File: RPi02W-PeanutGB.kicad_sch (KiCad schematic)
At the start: 64 parts, among them J1 Raspberry_Pi_2_3, J3 AudioJack3_SwitchTR, J4 Conn_01x50, J5 Conn_02x10_Odd_Even, J6 Conn_02x10_Odd_Even, J7 Conn_02x10_Odd_Even, J8 Conn_02x10_Odd_Even, J9 USB_C_Receptacle, SW1 SW_SPDT_MSM, SW10 SW_Push, SW11 SW_Push, SW12 SW_Push, SW13 SW_Push, SW14 SW_Push, SW2 SW_Push, SW3 SW_Push, SW4 SW_Push, SW5 SW_Push, SW6 SW_Push, SW7 SW_Push, SW8 SW_Push, SW9 SW_Push, U1 MCP73831-2-OT, U3 LM4861MX

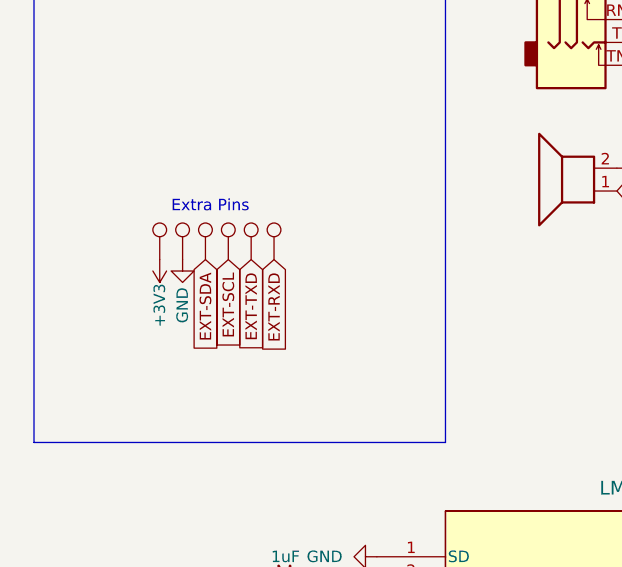
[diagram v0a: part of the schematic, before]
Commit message: Add files via upload
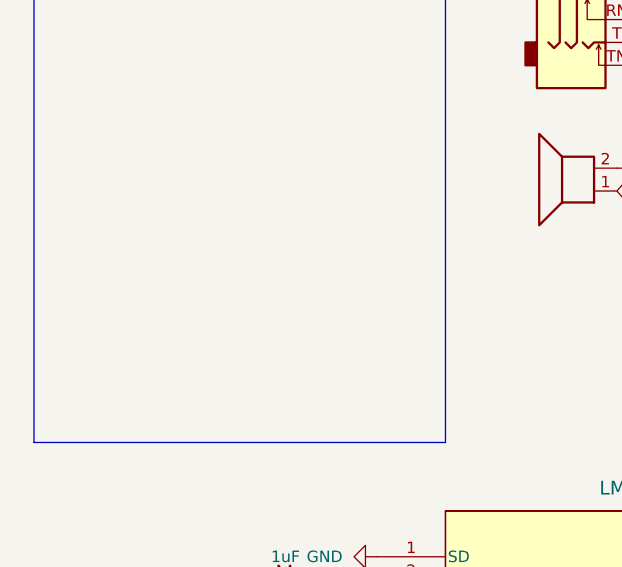
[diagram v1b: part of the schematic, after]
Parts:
- removed TP10, TP11, TP12, TP5, TP7, TP9: TestPoint, RPi02W-PeanutGB:TestPoint_THTPad_Edit_D1.5mm_Drill0.7mm, symbol Connector:TestPoint
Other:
- note removed: "Extra Pins"
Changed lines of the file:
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@@
     (effects (font (size 1.27 1.27)) (justify left bottom))
   )
-  (text "Extra Pins" (at 33.02 83.82 0)
-    (effects (font (size 1.27 1.27)) (justify left bottom))
-  )
   (global_label "BUTTON-DR" (shape input) (at 118.11 171.45 0) (fields_autoplaced)
     (effects (font (size 1.27 1.27)) (justify left))
@@
     )
   )
-  (global_label "EXT-SDA" (shape input) (at 36.83 88.9 270) (fields_autoplaced)
-    (effects (font (size 1.27 1.27)) (justify right))
-    (property "Intersheetrefs" "${INTERSHEET_REFS}" (at 36.83 100.3518 90)
-      (effects (font (size 1.27 1.27)) (justify right) hide)
-    )
-  )
   (global_label "BUTTON-B" (shape input) (at 195.58 22.86 0) (fields_autoplaced)
     (effects (font (size 1.27 1.27)) (justify left))
@@
     )
   )
-  (global_label "EXT-TXD" (shape input) (at 41.91 88.9 270) (fields_autoplaced)
-    (effects (font (size 1.27 1.27)) (justify right))
-    (property "Intersheetrefs" "${INTERSHEET_REFS}" (at 41.91 100.2308 90)
-      (effects (font (size 1.27 1.27)) (justify right) hide)
-    )
-  )
   (global_label "LCD-MOSI" (shape input) (at 217.17 181.61 180) (fields_autoplaced)
     (effects (font (size 1.27 1.27)) (justify right))
@@
     )
   )
-  (global_label "EXT-RXD" (shape input) (at 44.45 88.9 270) (fields_autoplaced)
-    (effects (font (size 1.27 1.27)) (justify right))
-    (property "Intersheetrefs" "${INTERSHEET_REFS}" (at 44.45 100.5332 90)
-      (effects (font (size 1.27 1.27)) (justify right) hide)
-    )
-  )
   (global_label "AUDIO-SPEAKER" (shape input) (at 82.55 81.28 0) (fields_autoplaced)
     (effects (font (size 1.27 1.27)) (justify left))
@@
     )
   )
-  (global_label "EXT-SCL" (shape input) (at 39.37 88.9 270) (fields_autoplaced)
-    (effects (font (size 1.27 1.27)) (justify right))
-    (property "Intersheetrefs" "${INTERSHEET_REFS}" (at 39.37 100.2913 90)
-      (effects (font (size 1.27 1.27)) (justify right) hide)
-    )
-  )
   (global_label "BUTTON-DL" (shape input) (at 57.15 171.45 180) (fields_autoplaced)
     (effects (font (size 1.27 1.27)) (justify right))
@@
     (property "Intersheetrefs" "${INTERSHEET_REFS}" (at 202.8757 176.53 0)
       (effects (font (size 1.27 1.27)) (justify right) hide)
-    )
-  )
-  (symbol (lib_id "Connector:TestPoint") (at 44.45 88.9 0) (unit 1)
-    (in_bom yes) (on_board yes) (dnp no) (fields_autoplaced)
-    (property "Reference" "TP12" (at 46.99 84.328 0)
-      (effects (font (size 1.27 1.27)) (justify left) hide)
-    )
-    (property "Value" "TestPoint" (at 46.99 86.868 0)
-      (effects (font (size 1.27 1.27)) (justify left) hide)
-    )
-    (property "Footprint" "RPi02W-PeanutGB:TestPoint_THTPad_Edit_D1.5mm_Drill0.7mm" (at 49.53 88.9 0)
-      (effects (font (size 1.27 1.27)) hide)
-    )
-    (property "Datasheet" "~" (at 49.53 88.9 0)
-      (effects (font (size 1.27 1.27)) hide)
-    )
-    (pin "1")
-    (instances
-      (project "RPi02W-PeanutGB"
-        (path "/4ab622d7-b3cd-4c8b-9519-077cc9b8f532"
-          (reference "TP12") (unit 1)
-        )
-      )
-    )
-  )
-  (symbol (lib_id "Connector:TestPoint") (at 31.75 88.9 0) (unit 1)
-    (in_bom yes) (on_board yes) (dnp no) (fields_autoplaced)
-    (property "Reference" "TP5" (at 34.29 84.328 0)
-      (effects (font (size 1.27 1.27)) (justify left) hide)
-    )
-    (property "Value" "TestPoint" (at 34.29 86.868 0)
-      (effects (font (size 1.27 1.27)) (justify left) hide)
-    )
-    (property "Footprint" "RPi02W-PeanutGB:TestPoint_THTPad_Edit_D1.5mm_Drill0.7mm" (at 36.83 88.9 0)
-      (effects (font (size 1.27 1.27)) hide)
-    )
-    (property "Datasheet" "~" (at 36.83 88.9 0)
-      (effects (font (size 1.27 1.27)) hide)
-    )
-    (pin "1")
-    (instances
-      (project "RPi02W-PeanutGB"
-        (path "/4ab622d7-b3cd-4c8b-9519-077cc9b8f532"
-          (reference "TP5") (unit 1)
-        )
-      )
     )
   )
@@
         (path "/4ab622d7-b3cd-4c8b-9519-077cc9b8f532"
           (reference "#PWR01") (unit 1)
-        )
-      )
-    )
-  )
-  (symbol (lib_id "Connector:TestPoint") (at 41.91 88.9 0) (unit 1)
-    (in_bom yes) (on_board yes) (dnp no) (fields_autoplaced)
-    (property "Reference" "TP11" (at 44.45 84.328 0)
-      (effects (font (size 1.27 1.27)) (justify left) hide)
-    )
-    (property "Value" "TestPoint" (at 44.45 86.868 0)
-      (effects (font (size 1.27 1.27)) (justify left) hide)
-    )
-    (property "Footprint" "RPi02W-PeanutGB:TestPoint_THTPad_Edit_D1.5mm_Drill0.7mm" (at 46.99 88.9 0)
-      (effects (font (size 1.27 1.27)) hide)
-    )
-    (property "Datasheet" "~" (at 46.99 88.9 0)
-      (effects (font (size 1.27 1.27)) hide)
-    )
-    (pin "1")
-    (instances
-      (project "RPi02W-PeanutGB"
-        (path "/4ab622d7-b3cd-4c8b-9519-077cc9b8f532"
-          (reference "TP11") (unit 1)
         )
       )
@@
     )
   )
-  (symbol (lib_id "Connector:TestPoint") (at 34.29 88.9 0) (unit 1)
-    (in_bom yes) (on_board yes) (dnp no) (fields_autoplaced)
-    (property "Reference" "TP7" (at 36.83 84.328 0)
-      (effects (font (size 1.27 1.27)) (justify left) hide)
-    )
-    (property "Value" "TestPoint" (at 36.83 86.868 0)
-      (effects (font (size 1.27 1.27)) (justify left) hide)
-    )
-    (property "Footprint" "RPi02W-PeanutGB:TestPoint_THTPad_Edit_D1.5mm_Drill0.7mm" (at 39.37 88.9 0)
-      (effects (font (size 1.27 1.27)) hide)
-    )
-    (property "Datasheet" "~" (at 39.37 88.9 0)
-      (effects (font (size 1.27 1.27)) hide)
-    )
-    (pin "1")
-    (instances
-      (project "RPi02W-PeanutGB"
-        (path "/4ab622d7-b3cd-4c8b-9519-077cc9b8f532"
-          (reference "TP7") (unit 1)
-        )
-      )
-    )
-  )
   (symbol (lib_id "Device:R_US") (at 247.65 35.56 90) (unit 1)
     (in_bom yes) (on_board yes) (dnp no)
@@
         (path "/4ab622d7-b3cd-4c8b-9519-077cc9b8f532"
           (reference "R8") (unit 1)
-        )
-      )
-    )
-  )
-  (symbol (lib_id "Connector:TestPoint") (at 39.37 88.9 0) (unit 1)
-    (in_bom yes) (on_board yes) (dnp no) (fields_autoplaced)
-    (property "Reference" "TP10" (at 41.91 84.328 0)
-      (effects (font (size 1.27 1.27)) (justify left) hide)
-    )
-    (property "Value" "TestPoint" (at 41.91 86.868 0)
-      (effects (font (size 1.27 1.27)) (justify left) hide)
-    )
-    (property "Footprint" "RPi02W-PeanutGB:TestPoint_THTPad_Edit_D1.5mm_Drill0.7mm" (at 44.45 88.9 0)
-      (effects (font (size 1.27 1.27)) hide)
-    )
-    (property "Datasheet" "~" (at 44.45 88.9 0)
-      (effects (font (size 1.27 1.27)) hide)
-    )
-    (pin "1")
-    (instances
-      (project "RPi02W-PeanutGB"
-        (path "/4ab622d7-b3cd-4c8b-9519-077cc9b8f532"
-          (reference "TP10") (unit 1)
         )
       )
@@
     )
   )
-  (symbol (lib_id "Connector:TestPoint") (at 36.83 88.9 0) (unit 1)
-    (in_bom yes) (on_board yes) (dnp no) (fields_autoplaced)
-    (property "Reference" "TP9" (at 39.37 84.328 0)
-      (effects (font (size 1.27 1.27)) (justify left) hide)
-    )
-    (property "Value" "TestPoint" (at 39.37 86.868 0)
-      (effects (font (size 1.27 1.27)) (justify left) hide)
-    )
-    (property "Footprint" "RPi02W-PeanutGB:TestPoint_THTPad_Edit_D1.5mm_Drill0.7mm" (at 41.91 88.9 0)
-      (effects (font (size 1.27 1.27)) hide)
-    )
-    (property "Datasheet" "~" (at 41.91 88.9 0)
-      (effects (font (size 1.27 1.27)) hide)
-    )
-    (pin "1")
-    (instances
-      (project "RPi02W-PeanutGB"
-        (path "/4ab622d7-b3cd-4c8b-9519-077cc9b8f532"
-          (reference "TP9") (unit 1)
-        )
-      )
-    )
-  )
   (symbol (lib_id "power:+3V3") (at 118.11 163.83 270) (unit 1)
     (in_bom yes) (on_board yes) (dnp no)
@@
         )
       )
-    )
-  )
-  (symbol (lib_id "power:GND") (at 34.29 88.9 0) (unit 1)
-    (in_bom yes) (on_board yes) (dnp no)
-    (property "Reference" "#PWR071" (at 34.29 95.25 0)
-      (effects (font (size 1.27 1.27)) hide)
-    )
-    (property "Value" "GND" (at 34.29 93.98 90)
-      (effects (font (size 1.27 1.27)))
-    )
-    (property "Footprint" "" (at 34.29 88.9 0)
-      (effects (font (size 1.27 1.27)) hide)
-    )
-    (property "Datasheet" "" (at 34.29 88.9 0)
-      (effects (font (size 1.27 1.27)) hide)
-    )
-    (pin "1")
-    (instances
-      (project "RPi02W-PeanutGB"
-        (path "/4ab622d7-b3cd-4c8b-9519-077cc9b8f532"
-          (reference "#PWR071") (unit 1)
-        )
-      )
-    )
-  )
-  (symbol (lib_id "power:+3V3") (at 31.75 88.9 180) (unit 1)
-    (in_bom yes) (on_board yes) (dnp no)
-    (property "Reference" "#PWR070" (at 31.75 85.09 0)
-      (effects (font (size 1.27 1.27)) hide)
-    )
-    (property "Value" "+3V3" (at 31.75 93.98 90)
-      (effects (font (size 1.27 1.27)))
-    )
-    (property "Footprint" "" (at 31.75 88.9 0)
-      (effects (font (size 1.27 1.27)) hide)
-    )
-    (property "Datasheet" "" (at 31.75 88.9 0)
-      (effects (font (size 1.27 1.27)) hide)
-    )
-    (pin "1")
-    (instances
-      (project "RPi02W-PeanutGB"
-        (path "/4ab622d7-b3cd-4c8b-9519-077cc9b8f532"
-          (reference "#PWR070") (unit 1)
-        )
-      )

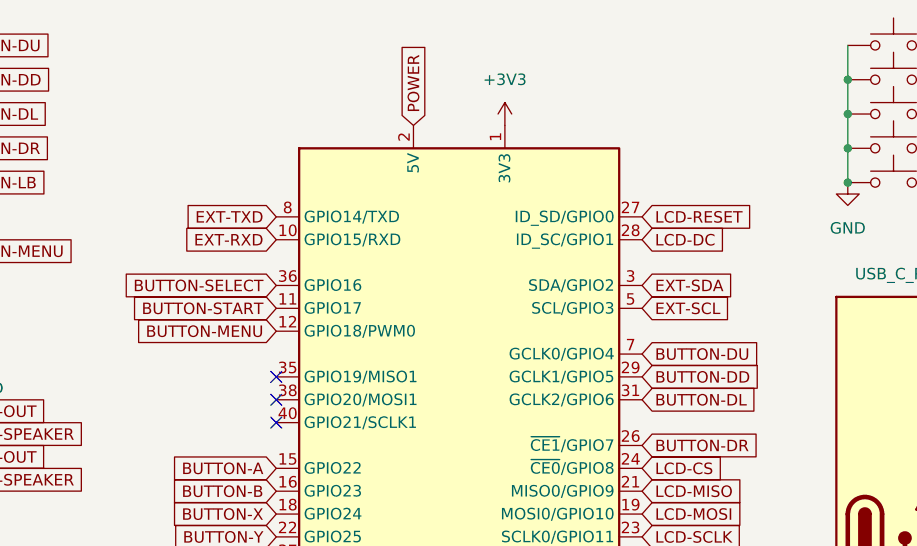
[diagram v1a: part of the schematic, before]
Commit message: Add files via upload
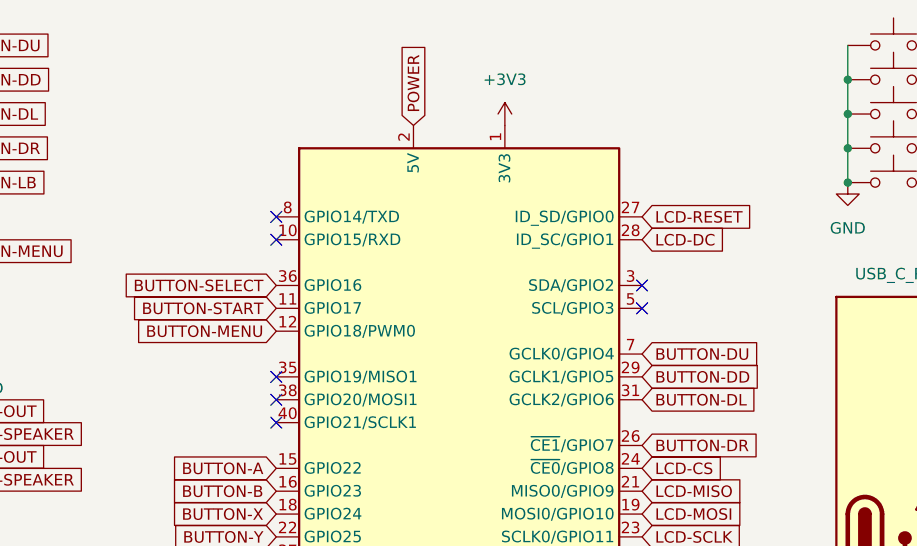
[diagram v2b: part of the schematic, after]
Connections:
- net EXT-RXD: no longer names the net of J1.10 (GPIO15/RXD)
- net EXT-SCL: no longer names the net of J1.5 (SCL/GPIO3)
- net EXT-SDA: no longer names the net of J1.3 (SDA/GPIO2)
- net EXT-TXD: no longer names the net of J1.8 (GPIO14/TXD)
- no-connect marks 44 -> 48
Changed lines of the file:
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@@
   (no_connect (at 209.55 97.79))
   (no_connect (at 105.41 184.15))
+  (no_connect (at 121.92 40.64))
   (no_connect (at 209.55 64.77))
   (no_connect (at 121.92 60.96))
@@
   (no_connect (at 118.11 184.15))
   (no_connect (at 229.87 176.53))
+  (no_connect (at 162.56 45.72))
   (no_connect (at 167.64 186.69))
   (no_connect (at 209.55 62.23))
@@
   (no_connect (at 118.11 181.61))
   (no_connect (at 209.55 105.41))
+  (no_connect (at 121.92 38.1))
   (no_connect (at 57.15 186.69))
   (no_connect (at 209.55 69.85))
   (no_connect (at 209.55 107.95))
   (no_connect (at 69.85 179.07))
+  (no_connect (at 162.56 48.26))
   (no_connect (at 69.85 186.69))
   (no_connect (at 69.85 184.15))
@@
     )
   )
-  (global_label "EXT-SDA" (shape input) (at 162.56 45.72 0) (fields_autoplaced)
-    (effects (font (size 1.27 1.27)) (justify left))
-    (property "Intersheetrefs" "${INTERSHEET_REFS}" (at 174.0118 45.72 0)
-      (effects (font (size 1.27 1.27)) (justify left) hide)
-    )
-  )
   (global_label "LCD-RESET" (shape input) (at 167.64 184.15 180) (fields_autoplaced)
     (effects (font (size 1.27 1.27)) (justify right))
@@
     )
   )
-  (global_label "EXT-RXD" (shape input) (at 121.92 40.64 180) (fields_autoplaced)
-    (effects (font (size 1.27 1.27)) (justify right))
-    (property "Intersheetrefs" "${INTERSHEET_REFS}" (at 110.2868 40.64 0)
-      (effects (font (size 1.27 1.27)) (justify right) hide)
-    )
-  )
   (global_label "BUTTON-SELECT" (shape input) (at 167.64 173.99 180) (fields_autoplaced)
     (effects (font (size 1.27 1.27)) (justify right))
@@
     )
   )
-  (global_label "EXT-SCL" (shape input) (at 162.56 48.26 0) (fields_autoplaced)
-    (effects (font (size 1.27 1.27)) (justify left))
-    (property "Intersheetrefs" "${INTERSHEET_REFS}" (at 173.9513 48.26 0)
-      (effects (font (size 1.27 1.27)) (justify left) hide)
-    )
-  )
   (global_label "BUTTON-RB" (shape input) (at 121.92 78.74 180) (fields_autoplaced)
     (effects (font (size 1.27 1.27)) (justify right))
@@
       (effects (font (size 1.27 1.27)) (justify right) hide)
     )
-  )
-  (global_label "EXT-TXD" (shape input) (at 121.92 38.1 180) (fields_autoplaced)
-    (effects (font (size 1.27 1.27)) (justify right))
-    (property "Intersheetrefs" "${INTERSHEET_REFS}" (at 110.5892 38.1 0)
-      (effects (font (size 1.27 1.27)) (justify right) hide)
-    )
